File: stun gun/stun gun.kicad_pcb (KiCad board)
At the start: 2 copper layers, 68.6 x 53.3 mm, 17 parts, among them J1 Power, J2 Digital/PWM, J3 Analog, J4 Digital/PWM, T1 Transformer_1P_1S, U1 LCD-016N002L

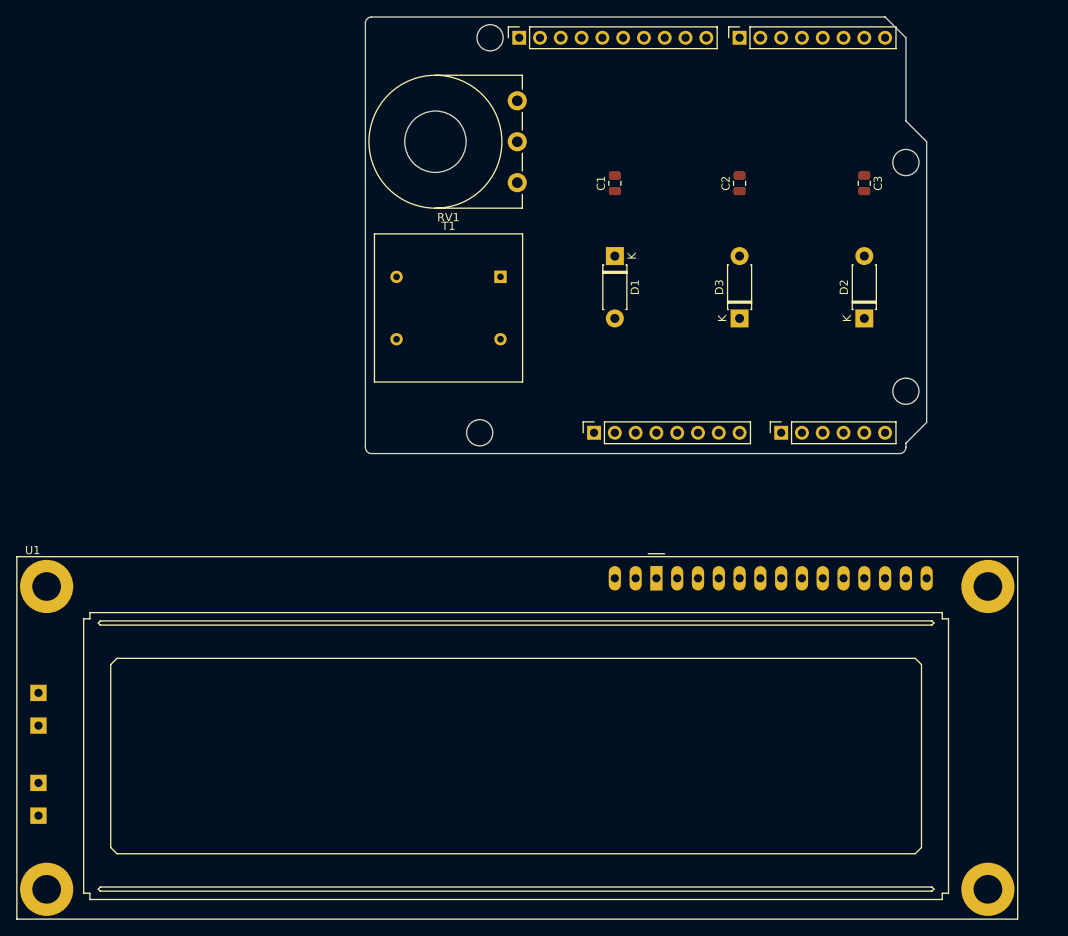
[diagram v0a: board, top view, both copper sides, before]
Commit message: Add files via upload
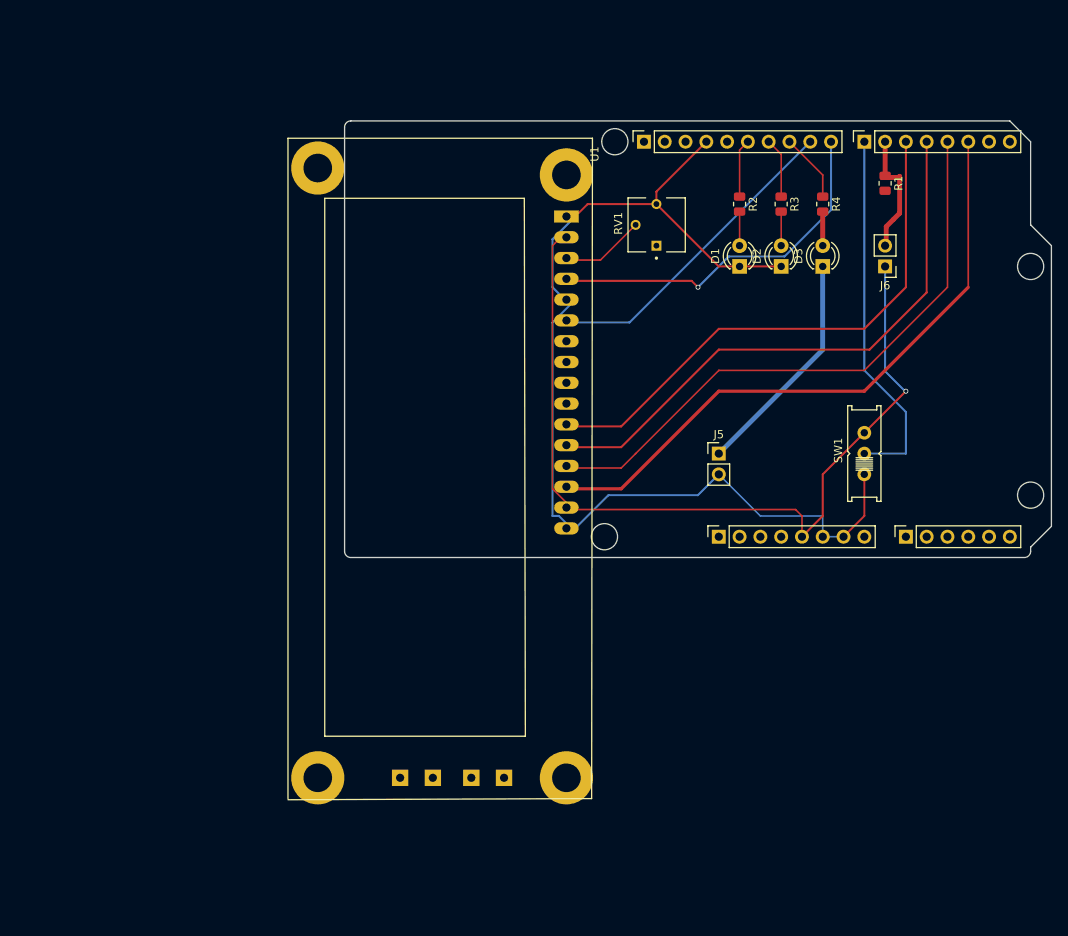
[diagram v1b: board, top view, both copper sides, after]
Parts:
- removed C1, C2: 1nF/3KV, Capacitor_SMD:C_0805_2012Metric
- removed C3: 1uF/3KV, Capacitor_SMD:C_0805_2012Metric
- removed T1: Transformer_1P_1S, Transformer_THT:Transformer_NF_ETAL_1-1_P1200
- added J5: Conn_01x02, Connector_PinHeader_2.54mm:PinHeader_1x02_P2.54mm_Vertical, F.Cu at (143.2, 100.0)
- added J6: Conn_01x02, Connector_PinHeader_2.54mm:PinHeader_1x02_P2.54mm_Vertical, F.Cu at (163.5, 77.1)
- added R1: 10K, Resistor_SMD:R_0805_2012Metric, F.Cu at (163.5, 67.0)
- added R2: 330, Resistor_SMD:R_0805_2012Metric, F.Cu at (145.7, 69.5)
- added R3: 330, Resistor_SMD:R_0805_2012Metric, F.Cu at (150.8, 69.5)
- added R4: 330, Resistor_SMD:R_0805_2012Metric, F.Cu at (155.9, 69.5)
- added SW1: SW_SPDT, slideswitch:EG1218, F.Cu at (161.0, 100.0)
- D1, D2, D3: value 1N4007 -> LED; footprint Diode_THT:D_DO-41_SOD81_P7.62mm_Horizontal -> LED_THT:LED_D3.0mm
- RV1: footprint Potentiometer_THT:Potentiometer_Piher_T-16L_Single_Vertical_Hole -> trimmer:TRIM_3362P-1-505LF
- moved U1 24.0 mm to (112.3, 109.5), turned to -90 degrees
- moved RV1 22.8 mm to (135.6, 72.1), turned to 90 degrees
- moved J1 19.8 mm to (143.2, 110.2)
- moved MH2 19.8 mm to (129.2, 110.2)
- moved MH3 19.8 mm to (181.3, 77.1)
- moved MH4 19.8 mm to (181.3, 105.1)
- moved J4 19.8 mm to (161.0, 61.9)
- moved J2 19.8 mm to (134.0, 61.9)
- moved MH1 19.8 mm to (130.5, 61.9)
- moved J3 19.8 mm to (166.0, 110.2)
- moved D1 15.3 mm to (145.7, 77.1), turned to 90 degrees
- moved D2 12.0 mm to (150.8, 77.1)
- moved D3 12.0 mm to (155.9, 77.1)
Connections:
- D1 pad 1: Net-(D1-Pad1) -> GND
- D2 pad 1: Net-(D2-Pad1) -> GND
- D2 pad 2: Net-(D1-Pad1) -> Net-(D2-Pad2)
- D3 pad 2: Net-(D2-Pad1) -> Net-(D3-Pad2)
- J1 pad 2: /IOREF -> unconnected-(J1-Pad2)
- J1 pad 3: /~{RESET} -> unconnected-(J1-Pad3)
- J1 pad 4: +3V3 -> unconnected-(J1-Pad4)
- J1 pad 8: VCC -> unconnected-(J1-Pad8)
- J2 pad 1: /SCL/A5 -> unconnected-(J2-Pad1)
- J2 pad 10: /8 -> /UNO_DP8
- J2 pad 2: /SDA/A4 -> unconnected-(J2-Pad2)
- J2 pad 3: /AREF -> unconnected-(J2-Pad3)
- J2 pad 5: /13 -> /UNO_DP13
- J2 pad 6: /12 -> /UNO_DP12
- J2 pad 7: /*11 -> /UNO_DP11
- J2 pad 8: /*10 -> /UNO_DP10
- J2 pad 9: /*9 -> /UNO_DP9
- J3 pad 1: /A0 -> unconnected-(J3-Pad1)
- J3 pad 2: /A1 -> unconnected-(J3-Pad2)
- J3 pad 3: /A2 -> unconnected-(J3-Pad3)
- J3 pad 4: /A3 -> unconnected-(J3-Pad4)
- J3 pad 5: /SDA/A4 -> unconnected-(J3-Pad5)
- J3 pad 6: /SCL/A5 -> unconnected-(J3-Pad6)
- J4 pad 1: /7 -> /UNO_DP7
- J4 pad 2: /*6 -> /UNO_DP6
- J4 pad 3: /*5 -> /UNO_DP5
- J4 pad 4: /4 -> /UNO_DP4
- J4 pad 5: /*3 -> /UNO_DP3
- J4 pad 6: /2 -> /UNO_DP2
- J4 pad 7: /TX/1 -> unconnected-(J4-Pad7)
- J4 pad 8: /RX/0 -> unconnected-(J4-Pad8)
- RV1 pad 1: +5V -> unconnected-(RV1-Pad1)
- U1 pad 11: /*10 -> /UNO_DP5
- U1 pad 12: /*11 -> /UNO_DP4
- U1 pad 13: /12 -> /UNO_DP3
- U1 pad 14: /13 -> /UNO_DP2
- U1 pad 15: +3V3 -> +5V
- U1 pad 4: /4 -> /UNO_DP8
- U1 pad 6: /6 -> /UNO_DP9
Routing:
- net GND: track 0.00 -> 131.8 mm
- net +5V: track 0.00 -> 106.4 mm, vias 0 -> 1
- net /UNO_DP2: track 0.00 -> 76.2 mm
- net /UNO_DP3: track 0.00 -> 72.6 mm
- net /UNO_DP4: track 0.00 -> 69.4 mm
- net /UNO_DP5: track 0.00 -> 65.5 mm
- net /UNO_DP7: track 0.00 -> 45.3 mm
- net /UNO_DP8: track 0.00 -> 44.1 mm, vias 0 -> 1
- net /UNO_DP9: track 0.00 -> 38.1 mm
- net Net-(D3-Pad1): track 0.00 -> 28.1 mm
- net /UNO_DP6: track 0.00 -> 14.8 mm
- net Net-(RV1-Pad2): track 0.00 -> 9.40 mm
- net /UNO_DP10: track 0.00 -> 8.39 mm
- net /UNO_DP11: track 0.00 -> 7.34 mm
- net /UNO_DP12: track 0.00 -> 7.13 mm
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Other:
- board size 68.6 x 53.3 mm -> 86.4 x 53.3 mm
- board text removed: "ICSP"
